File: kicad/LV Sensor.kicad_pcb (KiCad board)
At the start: 2 copper layers, 80.3 x 45.9 mm, 69 parts, among them IC1 MCP2517FDT-H_SL, IC2 L78L05ABUTR, IC3 TLV74133PDBVR, IC4 TLV74125PDBVR, IC5 MSPM0C1104SDGS20R, J1 Screw_Terminal_01x02, J16 USB_B_Micro, J2 Screw_Terminal_01x02, J3 Screw_Terminal_01x02, J4 Screw_Terminal_01x02, J5 Screw_Terminal_01x02, J6 43650-0401, SW1 SW_Push, U0 AP63205WU-7, U10 MCP3204-CI/P, U3 FT231XS-R, U6 DSC1001DL5-020.0000T, U7 ADS114S06BIPBSR, U8 LM2662MX/NOPB, U9 ATA6561-GAQW-N

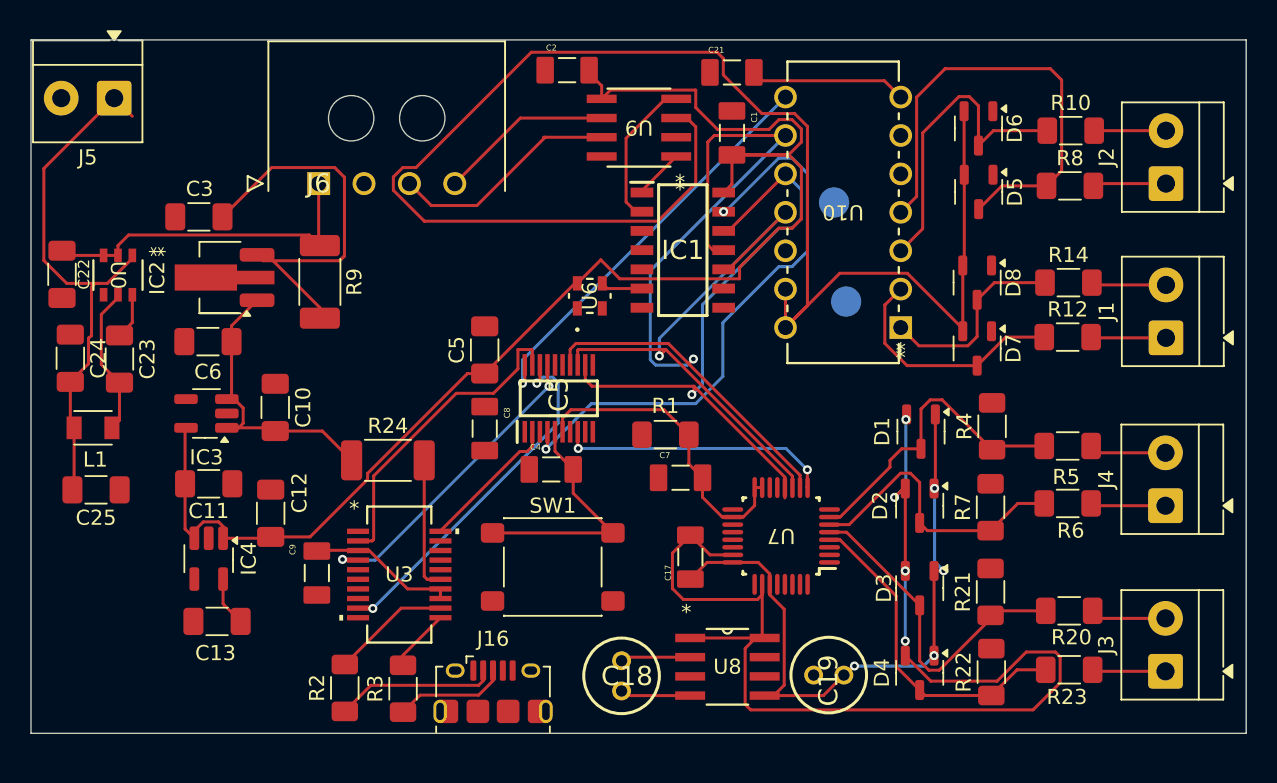
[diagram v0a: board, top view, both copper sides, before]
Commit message: Final Checks
Completed Board
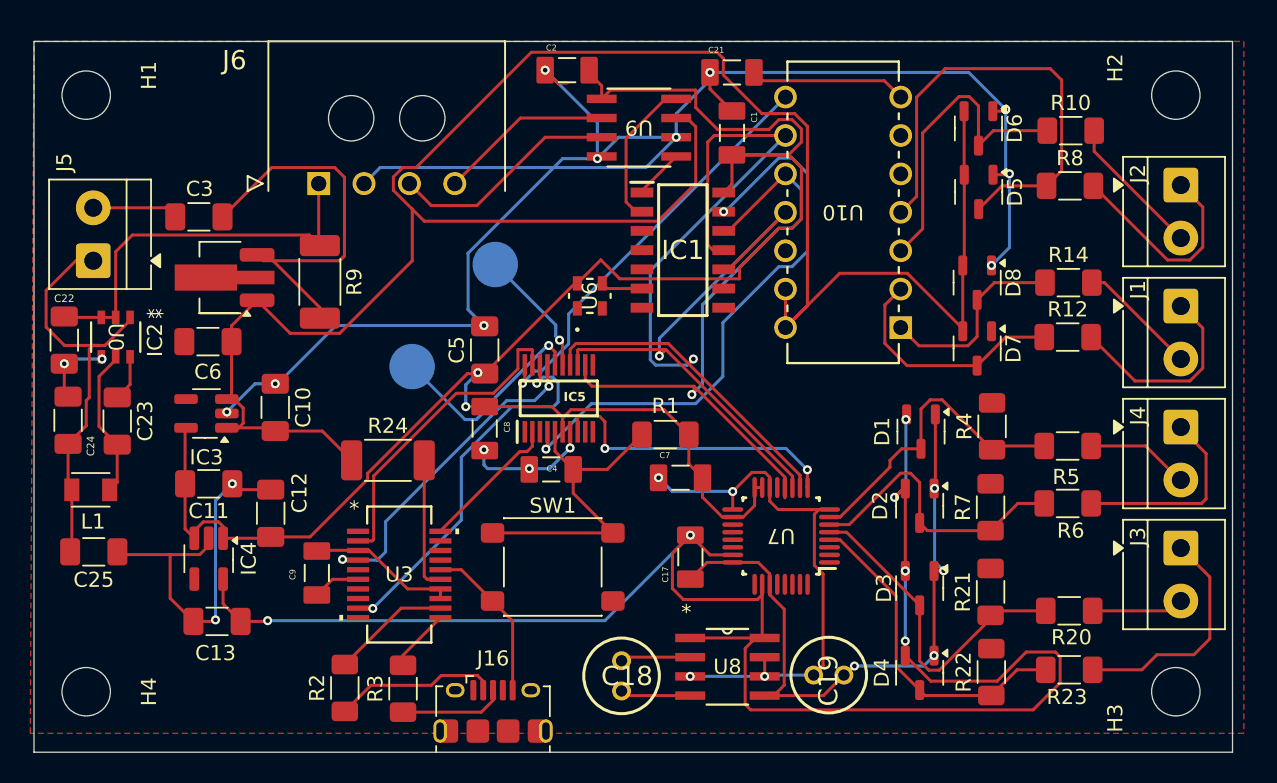
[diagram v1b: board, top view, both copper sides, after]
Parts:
- added H1: MountingHole, MountingHole:MountingHole_3.2mm_M3, F.Cu at (152.9, 55.8)
- added H2: MountingHole, MountingHole:MountingHole_3.2mm_M3, F.Cu at (225.0, 55.8)
- added H3: MountingHole, MountingHole:MountingHole_3.2mm_M3, F.Cu at (225.0, 95.2)
- added H4: MountingHole, MountingHole:MountingHole_3.2mm_M3, F.Cu at (152.9, 95.2)
- TP1, TP2: footprint TestPoint:TestPoint_Pad_D2.0mm -> TestPoint:TestPoint_Pad_D3.0mm
- moved TP1 29.9 mm to (174.5, 73.8)
- moved TP2 23.3 mm to (180.0, 67.0)
- moved J5 10.8 mm to (153.4, 66.8), turned to 90 degrees
- moved J3 8.21 mm to (225.3, 85.8), turned to -90 degrees
- moved J4 5.30 mm to (225.3, 77.8), turned to -90 degrees
- moved C22 4.35 mm to (151.5, 72.0)
- moved L1 4.10 mm to (153.2, 81.9)
- moved C23 4.10 mm to (155.0, 77.3)
- moved C24 4.10 mm to (151.8, 77.3)
- moved C25 4.10 mm to (153.4, 86.0)
- moved U0 4.10 mm to (154.9, 71.8)
- moved J1 2.32 mm to (225.3, 69.8), turned to -90 degrees
- moved J16 1.30 mm to (179.8, 96.5)
- moved J2 0.99 mm to (225.3, 61.8), turned to -90 degrees
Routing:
- net GND: track 0.00 -> 212.0 mm, vias 0 -> 22
- net +2V5: track 84.3 -> 116.4 mm, vias 4 -> 6
- net +5V: track 127.5 -> 144.0 mm
- net Net-(IC5-PA20_/_A6_/_SWCLK): track 0.00 -> 14.1 mm, vias 0 -> 1
- net Net-(J3-Pin_1): track 4.86 -> 15.5 mm
- net +3V3: track 116.3 -> 126.5 mm, vias 0 -> 2
- net Net-(J2-Pin_1): track 4.86 -> 14.5 mm
- net Net-(J1-Pin_1): track 4.97 -> 13.6 mm
- net /5V out: track 36.6 -> 28.1 mm
- net Net-(IC5-PA19_/_SWDIO): track 0.00 -> 8.48 mm, vias 0 -> 1
- net Net-(J4-Pin_1): track 4.98 -> 13.4 mm
- net Net-(IC5-PA1_/_NRST): track 16.2 -> 21.7 mm
- net Net-(J2-Pin_2): track 4.75 -> 9.47 mm
- net +12V: track 22.5 -> 26.6 mm
- net Net-(J1-Pin_2): track 4.96 -> 8.19 mm
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- added copper zone on F.Cu, net GND
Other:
- board size 80.3 x 45.9 mm -> 79.2 x 47 mm
- board text added: "- Manish Shrestha / Nov 2025"
